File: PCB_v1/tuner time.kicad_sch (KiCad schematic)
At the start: 16 parts

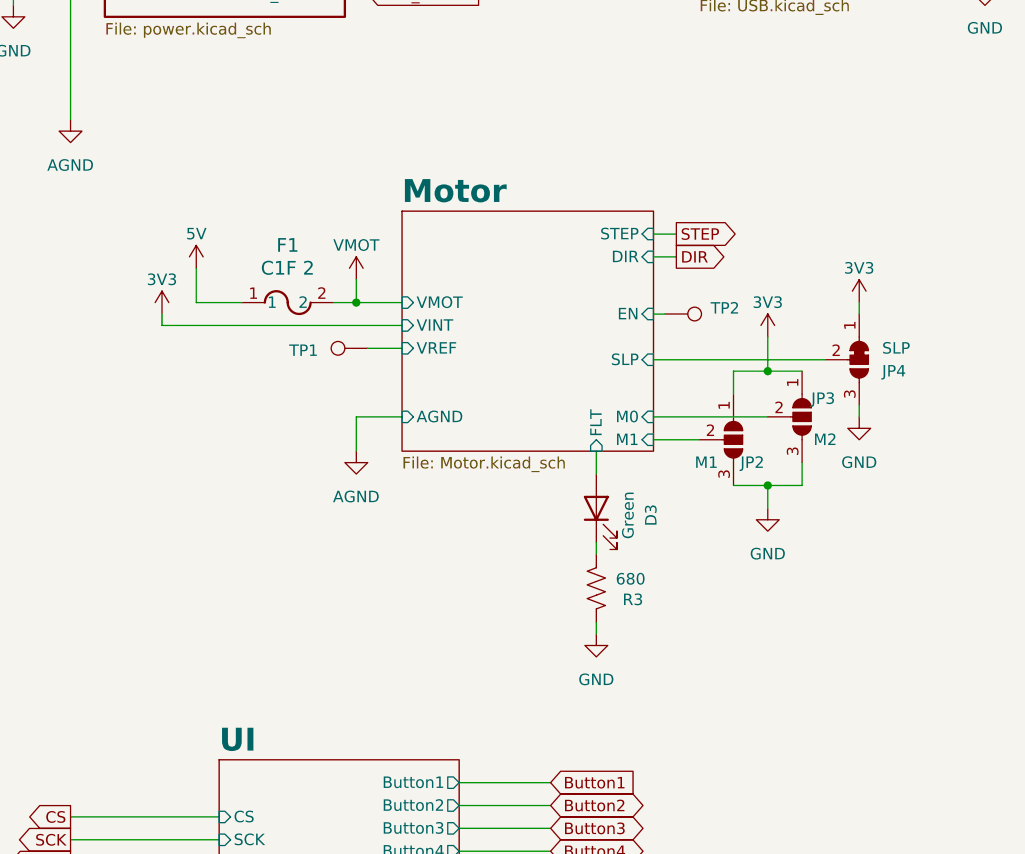
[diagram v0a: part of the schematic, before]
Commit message: before major move
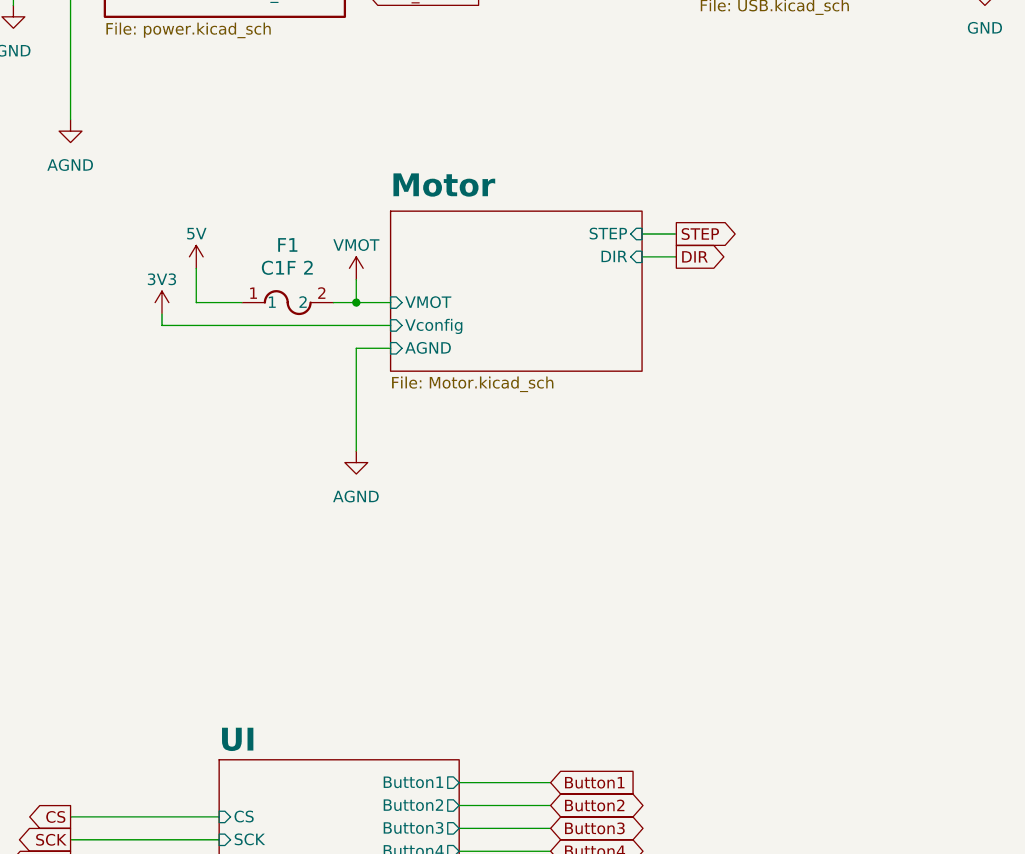
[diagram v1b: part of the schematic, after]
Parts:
- removed D3: Green, LED_0805_2012Metric_Pad1.15x1.40mm_HandSolder, symbol GT_LIbrary:LED
- removed JP2: M1, Jumper:SolderJumper-3_P1.3mm_Open_RoundedPad1.0x1.5mm, symbol GT_LIbrary:SolderJumper_3_Open
- removed JP3: M2, Jumper:SolderJumper-3_P1.3mm_Open_RoundedPad1.0x1.5mm, symbol GT_LIbrary:SolderJumper_3_Open
- removed JP4: SLP, Jumper:SolderJumper-3_P1.3mm_Bridged12_RoundedPad1.0x1.5mm, symbol GT_LIbrary:SolderJumper_3_Bridged12
- removed R3: 680, Resistor_SMD:R_0805_2012Metric, symbol GT_LIbrary:R_US
- removed TP1, TP2: ~, TestPoint_THTPad_D0.5mm_Drill0.3mm, symbol GT_LIbrary:TestPoint
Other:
- sheet Motor ports: added Vconfig; removed EN, FLT, M0, M1, SLP, VINT, VREF
